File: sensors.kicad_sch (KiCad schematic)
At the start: 5 parts, among them U701 TMP119AIYBGR, U702 INA226, U703 INA226

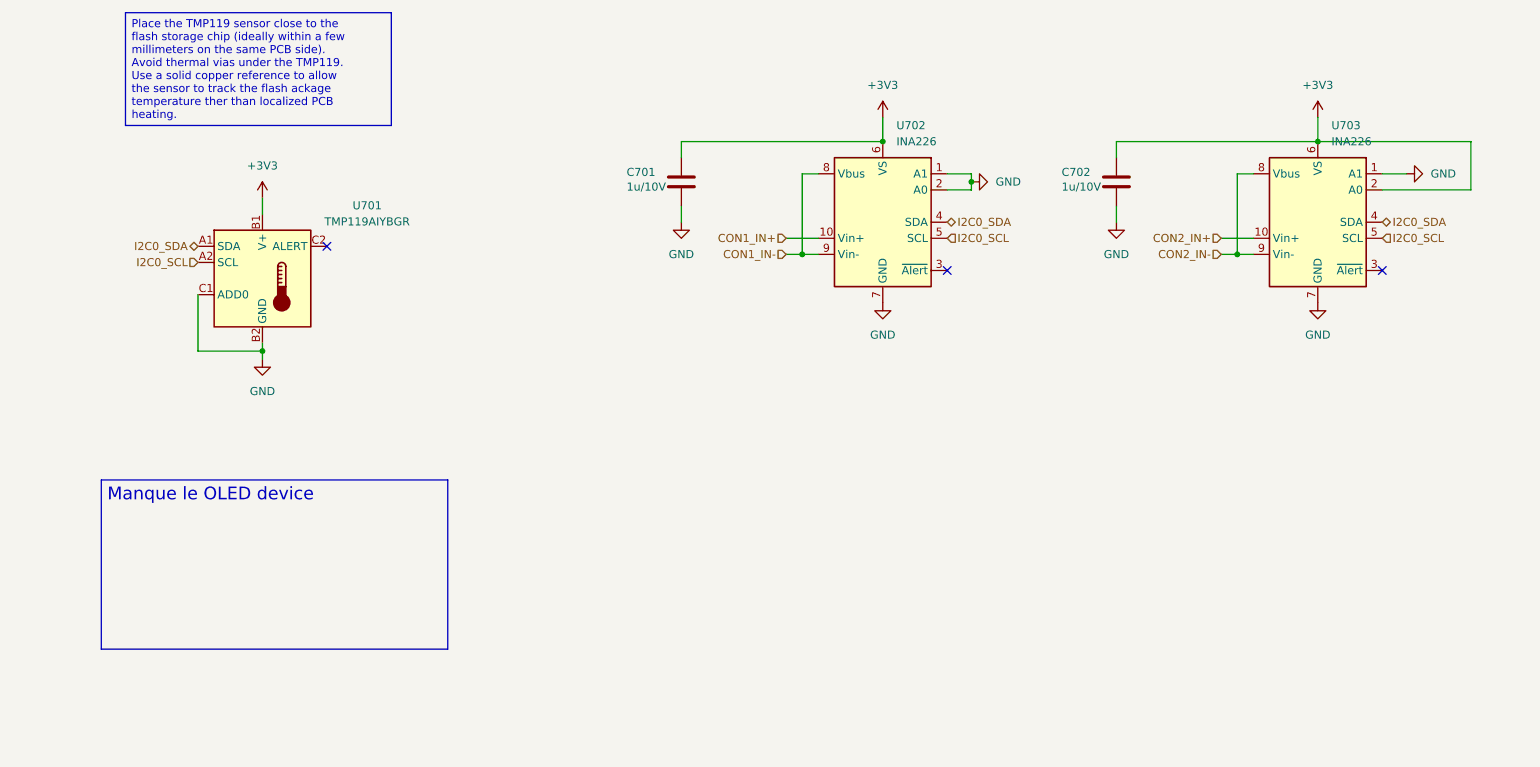
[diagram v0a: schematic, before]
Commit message: fin du schema et debut annotations precises
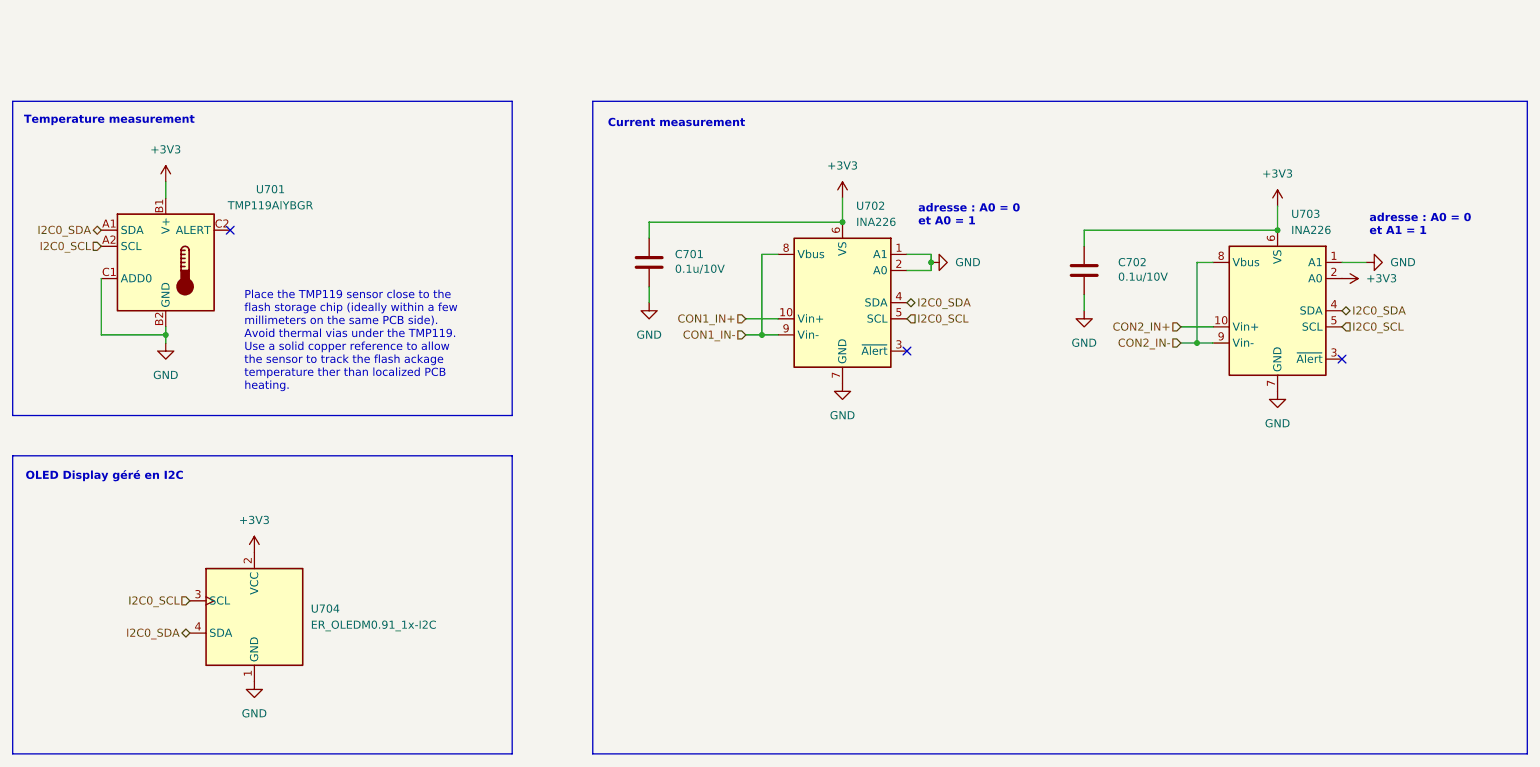
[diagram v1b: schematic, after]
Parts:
- added U704: ER_OLEDM0.91_1x-I2C, Display:ER_OLEDM0.91_1x-I2C, symbol Display_Graphic:ER_OLEDM0.91_1x-I2C
- C701, C702: value 1u/10V -> 0.1u/10V
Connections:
- net +3V3: now also U704.2 (VCC)
- net GND: now also U704.1 (GND)
- net I2C0_SCL: now also U704.3 (SCL)
- net I2C0_SDA: now also U704.4 (SDA)
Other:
- note added: "Current measurement"
- note added: "OLED Display géré en I2C"
- note added: "Temperature measurement"
- note added: "adresse : A0 = 0 et A0 = 1"
- note added: "adresse : A0 = 0 et A1 = 1"
- moved on the sheet: C701, C702, U701, U702, U703
